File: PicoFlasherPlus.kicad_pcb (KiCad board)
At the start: 2 copper layers, 35.6 x 61 mm, 4 parts, among them J1 1x7 Pin Header, SW1 SW_DIP_x01, U1 Pico, U2 TS3A27518EPW

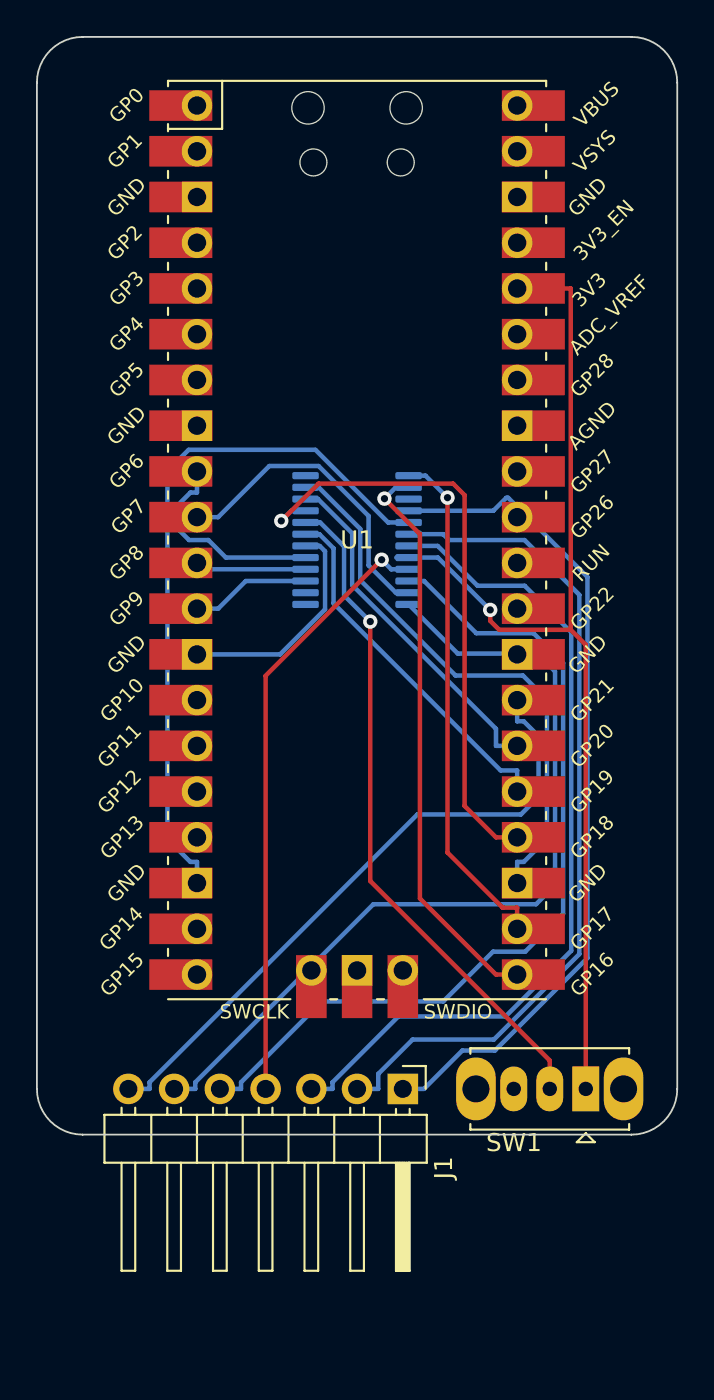
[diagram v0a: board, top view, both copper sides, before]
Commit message: Update
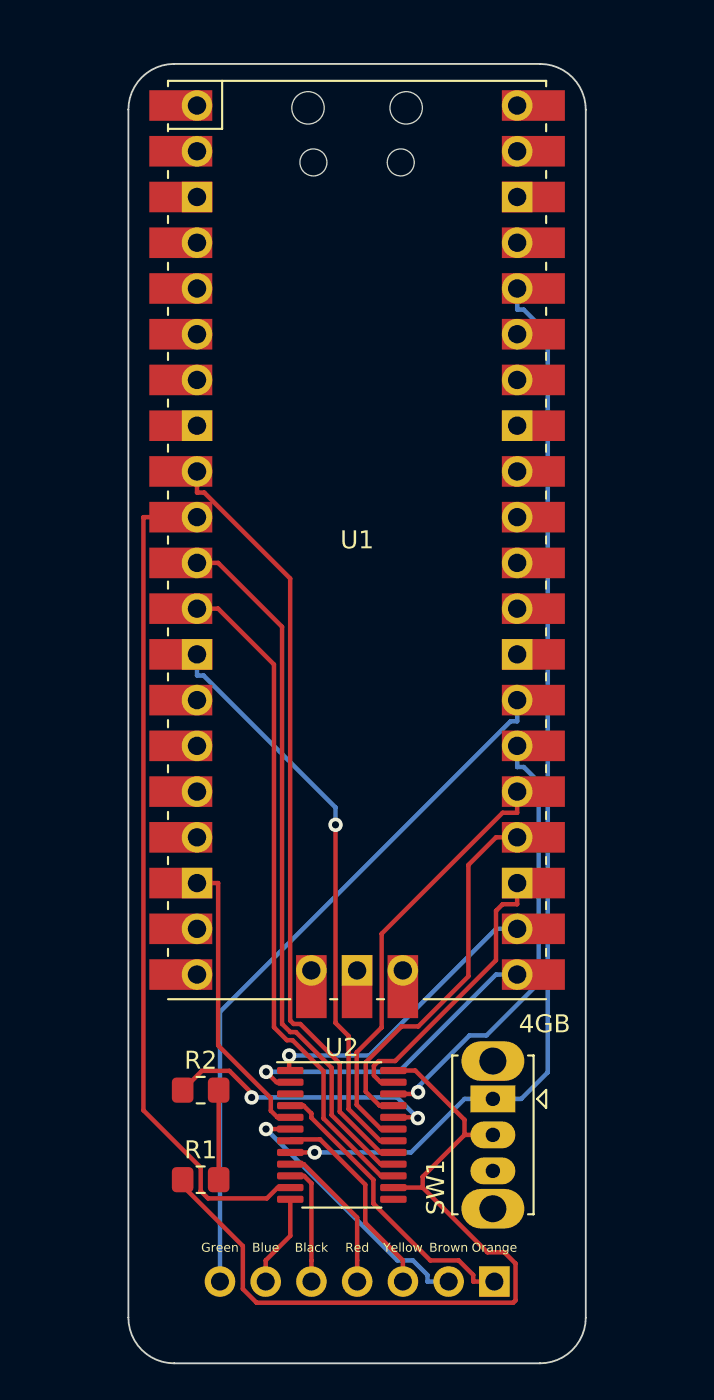
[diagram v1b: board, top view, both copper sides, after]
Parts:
- added R1: 10k, Resistor_SMD:R_0805_2012Metric_Pad1.20x1.40mm_HandSolder, F.Cu at (164.0, 109.2)
- added R2: 10k, Resistor_SMD:R_0805_2012Metric_Pad1.20x1.40mm_HandSolder, F.Cu at (164.0, 104.2)
- U2: moved to F.Cu
- moved U2 33.0 mm to (171.9, 106.7), turned to 0 degrees
- moved J1 11.8 mm to (180.3, 114.8)
- moved SW1 5.19 mm to (180.3, 104.7), turned to -90 degrees
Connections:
- SW1 pad 2: Net-(SW1-Pad2) -> Net-(R1-Pad1)
- U2 pad 14: unconnected-(U2-Pad14) -> Net-(R1-Pad1)
- U2 pad 20: Net-(SW1-Pad2) -> Net-(R2-Pad1)
- U2 pad 24: unconnected-(U2-Pad24) -> Net-(R1-Pad1)
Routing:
- net Net-(R1-Pad1): track 0.00 -> 44.9 mm
- net Net-(J1-Pad6): track 47.6 -> 5.14 mm
- net Net-(J1-Pad5): track 47.7 -> 6.80 mm
- net Net-(SW1-Pad2): track 37.5 -> 0.00 mm, vias 1 -> 0
- net Net-(J1-Pad3): track 46.5 -> 11.5 mm
- net Net-(U1-Pad11): track 6.17 -> 39.2 mm
- net Net-(J1-Pad2): track 46.8 -> 15.2 mm, vias 0 -> 1
- net Net-(U1-Pad9): track 11.7 -> 43.2 mm
- net Net-(U1-Pad12): track 6.66 -> 37.3 mm
- net Net-(J1-Pad1): track 46.5 -> 16.5 mm
- net Net-(U1-Pad10): track 17.5 -> 47.1 mm
- net Net-(J1-Pad4): track 33.8 -> 8.50 mm, vias 1 -> 0
- net Net-(U1-Pad18): track 39.3 -> 16.3 mm
- net Net-(U1-Pad13): track 12.6 -> 32.2 mm, vias 0 -> 1
- net Net-(R2-Pad1): track 0.00 -> 16.1 mm, vias 0 -> 2
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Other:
- board size 35.6 x 61 mm -> 25.4 x 72.2 mm
- board text added: "4GB"
- board text added: "Black"
- board text added: "Blue"
- board text added: "Brown"
- board text added: "Green"
- board text added: "Orange"
- board text added: "Red"
- board text added: "Yellow"
